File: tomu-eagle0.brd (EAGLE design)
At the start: 13.2 x 11.7 mm, 21 parts, among them U1 EFM32HG309F64G, X1 USBPCB

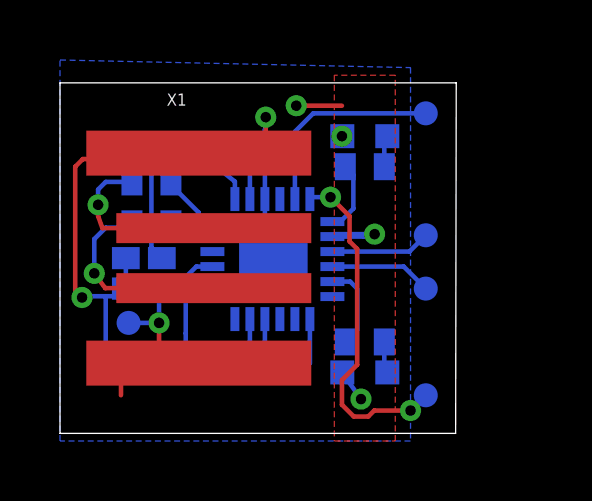
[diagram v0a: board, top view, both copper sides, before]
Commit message: added first pass at touch sensors
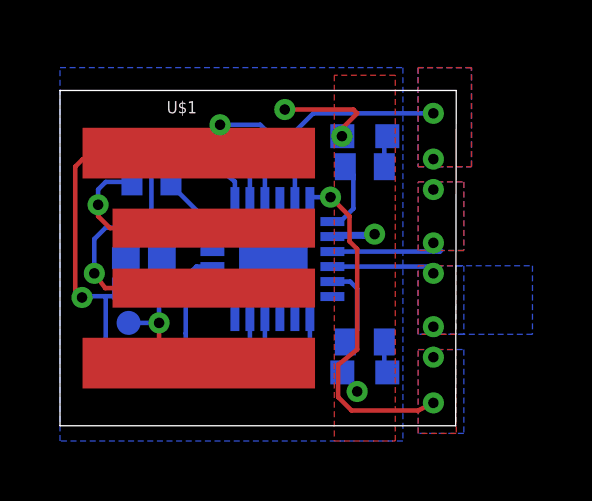
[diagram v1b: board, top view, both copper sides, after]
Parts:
- removed 0A, 0B, 1A, 1B: TPTP08R, testpad:TP08R
- removed X1: USBPCB, usb:USB-A-PCB
- added U$1: USBPCB2, todstuff:USB-A-PCB-2
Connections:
- net CAP0A: no longer 0A.TP
- net CAP0B: no longer 0B.TP
- net CAP1A: no longer 1A.TP
- net CAP1B: no longer 1B.TP
- net GND: now also U$1.GND; no longer X1.GND
- net USB_D+: now also U$1.USB_P; no longer X1.USB_P
- net USB_D-: now also U$1.USB_M; no longer X1.USB_M
- net VUSB: now also U$1.5V; no longer X1.5V
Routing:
- net VUSB: track 9.58 -> 6.93 mm
- net +3V3: track 9.24 -> 10.9 mm
- net GND: track 23.0 -> 22.4 mm
- net CAP0A: track 3.34 -> 3.63 mm, vias 0 -> 2
- net CAP0B: track 6.86 -> 7.12 mm, vias 0 -> 2
- net CAP1A: track 3.42 -> 3.39 mm, vias 0 -> 2
- net CAP1B: vias 2 -> 3
- added copper zone on layer 1, net CAP0A
- added copper zone on layer 16, net CAP0A
- added copper zone on layer 1, net CAP0B
- added copper zone on layer 16, net CAP0B
- added copper zone on layer 1, net CAP1A
- added copper zone on layer 16, net CAP1A
- added copper zone on layer 1, net CAP1B
- added copper zone on layer 16, net CAP1B
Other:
- board size 13.2 x 11.7 mm -> 13.2 x 11.2 mm
